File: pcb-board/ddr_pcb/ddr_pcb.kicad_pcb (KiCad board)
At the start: 2 copper layers, 65 x 65 mm, 13 parts, among them U1 RP2040_Zero

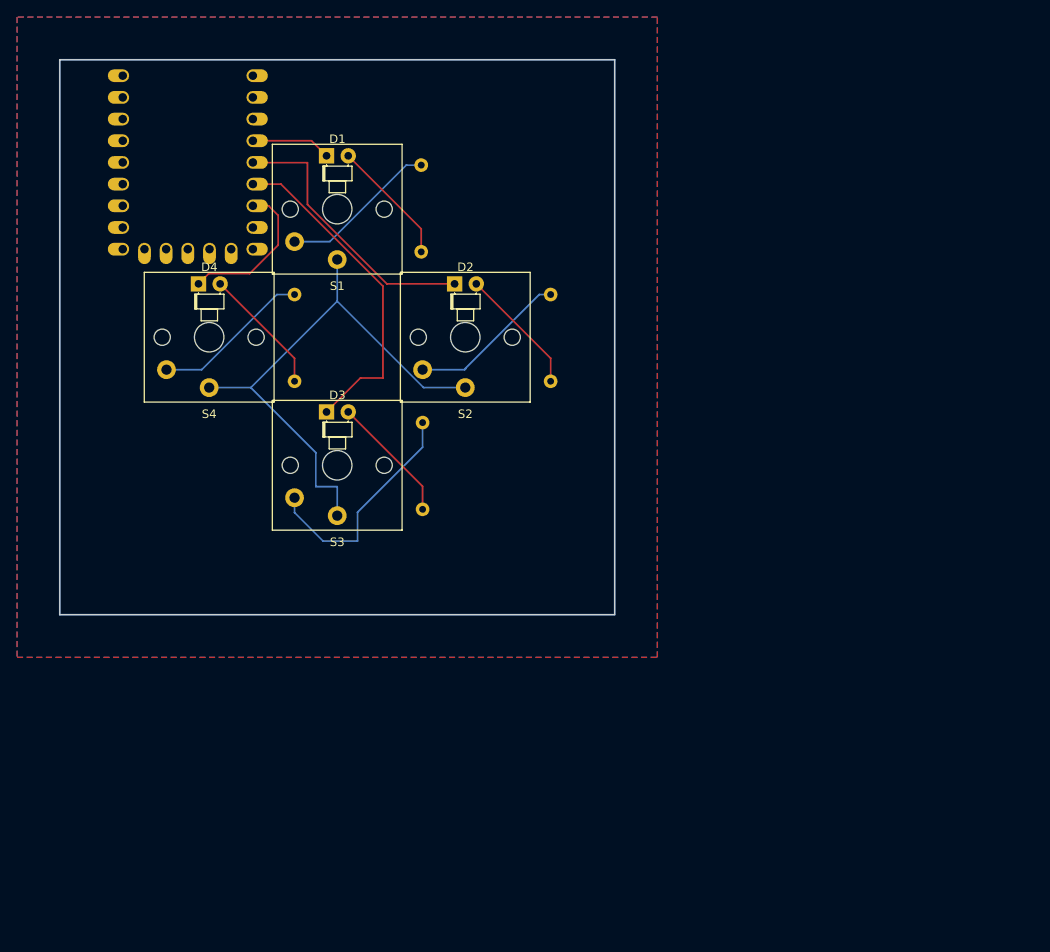
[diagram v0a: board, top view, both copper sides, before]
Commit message: like my 3rd pcb design
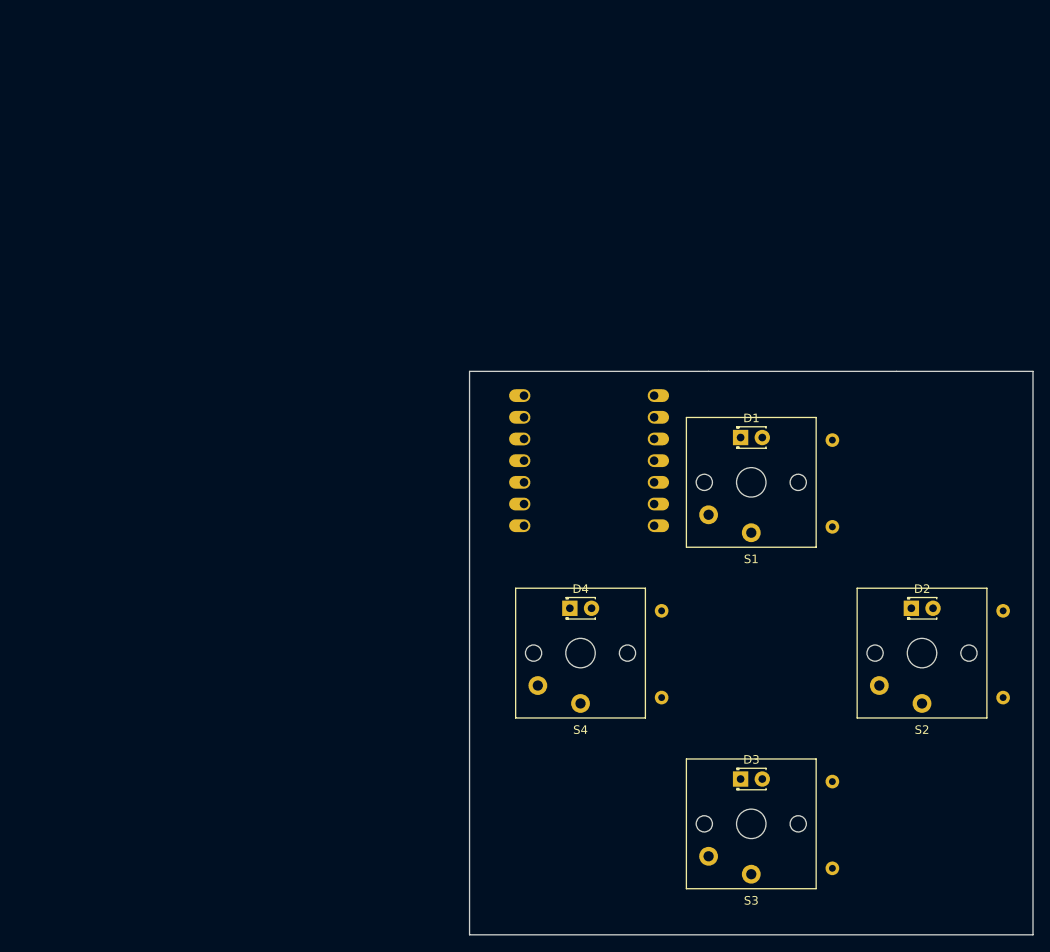
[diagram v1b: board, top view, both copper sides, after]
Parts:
- D1, D2, D3, D4: footprint LED_THT:LED_D1.8mm_W1.8mm_H2.4mm_Horizontal_O1.27mm_Z1.6mm -> LED_THT:LED_D1.8mm_W3.3mm_H2.4mm
- S1, S2, S3, S4: footprint ScottoKeebs_Choc:Choc_V1 -> ScottoKeebs_Choc:Choc_V1_1.00u
- moved D2 65.6 mm to (179.8, 84.2)
- moved S2 65.0 mm to (181.0, 89.5)
- moved D3 64.8 mm to (159.8, 104.2)
- moved S3 64.2 mm to (161.0, 109.5)
- moved U1 60.1 mm to (142.0, 69.5)
- moved R2 59.4 mm to (190.5, 84.5), turned to -90 degrees
- moved D1 58.7 mm to (159.8, 64.2)
- moved S1 58.1 mm to (161.0, 69.5)
- moved D4 57.8 mm to (139.8, 84.2)
- moved R3 57.6 mm to (170.5, 104.5), turned to -90 degrees
- moved S4 57.1 mm to (141.0, 89.5)
- moved R4 56.8 mm to (150.5, 94.7)
- moved R1 53.0 mm to (170.5, 64.5), turned to -90 degrees
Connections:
- D1 pad 1: UP -> GND
- D2 pad 1: RIGHT -> GND
- D3 pad 1: DOWN -> GND
- D4 pad 1: LEFT -> GND
- S1 pad 1: VCC -> UP
- S2 pad 1: VCC -> RIGHT
- S3 pad 1: VCC -> DOWN
- S4 pad 1: VCC -> LEFT
- U1 pad 22: unconnected-(U1-GND-Pad22) -> GND
- U1 pad 23: VCC -> unconnected-(U1-5V-Pad23)
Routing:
- net VCC: track 63.9 -> 0.00 mm
- net DOWN: track 39.2 -> 0.00 mm
- net RIGHT: track 32.4 -> 0.00 mm
- net Net-(R3-Pad2): track 27.5 -> 0.00 mm
- net Net-(R2-Pad2): track 18.7 -> 0.00 mm
- net Net-(R4-Pad2): track 18.6 -> 0.00 mm
- net Net-(R1-Pad2): track 18.6 -> 0.00 mm
- net LEFT: track 18.1 -> 0.00 mm
- net Net-(D2-A): track 15.0 -> 0.00 mm
- net Net-(D3-A): track 15.0 -> 0.00 mm
- net Net-(D4-A): track 15.0 -> 0.00 mm
- net Net-(D1-A): track 14.8 -> 0.00 mm
- net UP: track 9.36 -> 0.00 mm
- removed copper zone on B.Cu, net (none)
- removed copper zone on F.Cu, net (none)
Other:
- board size 65 x 65 mm -> 66 x 66 mm

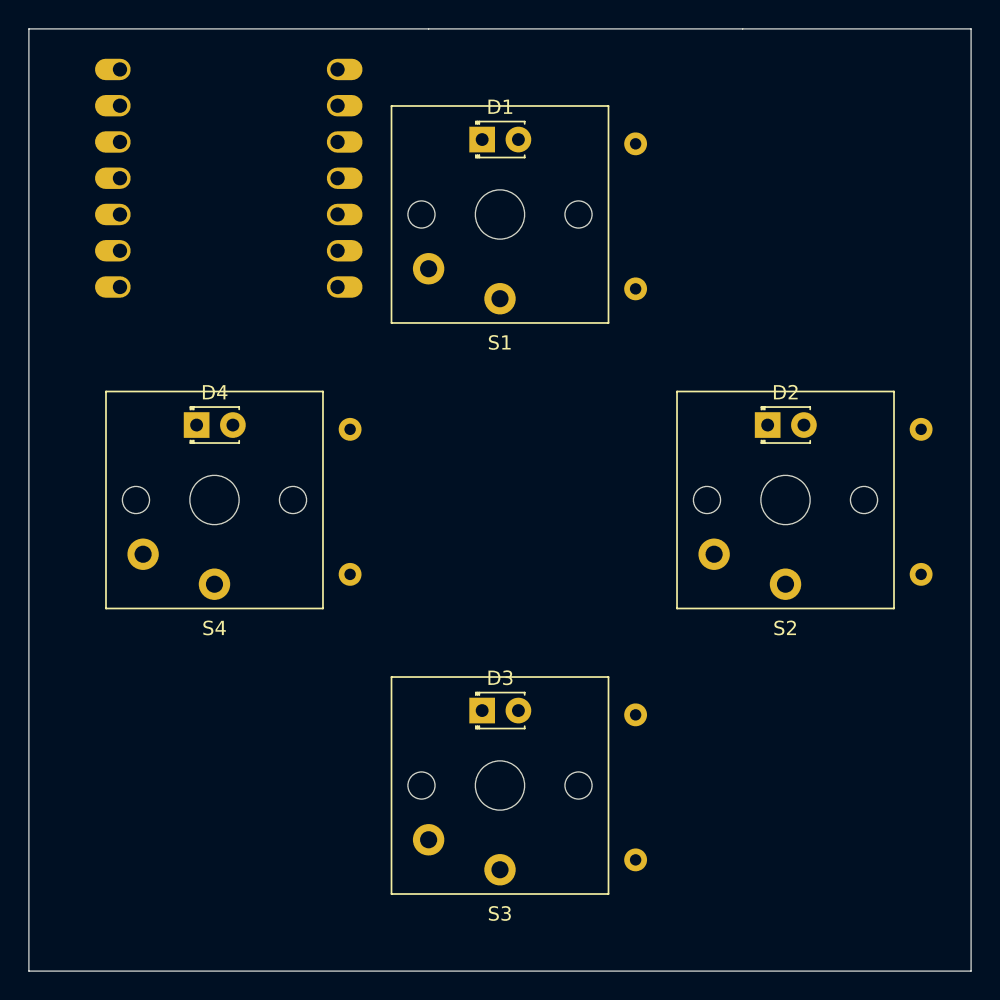
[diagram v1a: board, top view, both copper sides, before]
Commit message: starting code
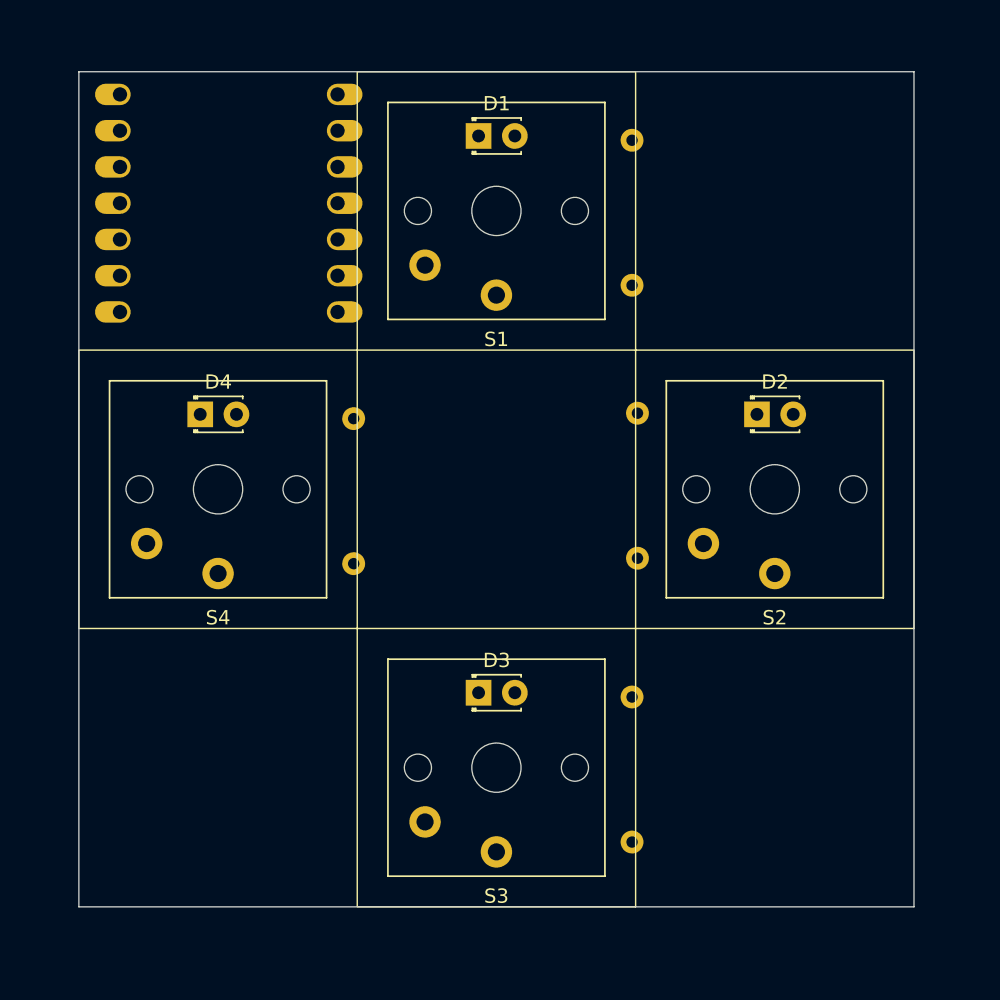
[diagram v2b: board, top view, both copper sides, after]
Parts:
- moved R2 19.9 mm to (170.6, 83.4)
- moved U1 1.75 mm to (142.0, 71.2)
- moved D3 1.27 mm to (159.5, 103.0)
- moved R3 1.27 mm to (170.2, 103.3)
- moved S3 1.27 mm to (160.8, 108.2)
- moved D2 1.06 mm to (179.0, 83.5)
- moved S2 1.06 mm to (180.2, 88.8)
- moved D4 0.79 mm to (140.0, 83.5)
- moved R4 0.79 mm to (150.8, 94.0)
- moved S4 0.79 mm to (141.2, 88.8)
- moved D1 0.35 mm to (159.5, 64.0)
- moved R1 0.35 mm to (170.2, 64.3)
- moved S1 0.35 mm to (160.8, 69.2)
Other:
- board size 66 x 66 mm -> 58.5 x 58.5 mm
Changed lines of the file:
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@@
 	(footprint "ScottoKeebs_Choc:Choc_V1_1.00u"
 		(layer "F.Cu")
-		(at 161 69.5 180)
+		(at 160.75 69.25 180)
 		(descr "Choc keyswitch V1 CPG1350 V1 Keycap 1.00u")
 		(tags "Choc Keyswitch Switch CPG1350 V1 Cutout Keycap 1.00u")
@@
 			(layer "F.SilkS")
 		)
-		(fp_line
-			(start 10 10)
-			(end 10 -10)
-			(stroke
-				(width 0.1)
-				(type solid)
-			)
-			(layer "Dwgs.User")
-		)
-		(fp_line
-			(start 10 -10)
-			(end -10 -10)
-			(stroke
-				(width 0.1)
-				(type solid)
-			)
-			(layer "Dwgs.User")
-		)
-		(fp_line
-			(start -10 10)
-			(end 10 10)
-			(stroke
-				(width 0.1)
-				(type solid)
-			)
-			(layer "Dwgs.User")
-		)
-		(fp_line
-			(start -10 -10)
-			(end -10 10)
+		(fp_rect
+			(start -9.75 -9.75)
+			(end 9.75 9.75)
 			(stroke
 				(width 0.1)
-				(type solid)
+				(type default)
 			)
-			(layer "Dwgs.User")
+			(fill none)
+			(layer "F.SilkS")
 		)
 		(fp_line
@@
 	(footprint "LED_THT:LED_D1.8mm_W3.3mm_H2.4mm"
 		(layer "F.Cu")
-		(at 139.75 84.25)
+		(at 140 83.5)
 		(descr "LED, Round,  Rectangular size 3.3x2.4mm^2 diameter 1.8mm, 2 pins")
 		(tags "LED Round  Rectangular size 3.3x2.4mm^2 diameter 1.8mm 2 pins")
@@
 	(footprint "LED_THT:LED_D1.8mm_W3.3mm_H2.4mm"
 		(layer "F.Cu")
-		(at 159.75 64.25)
+		(at 159.5 64)
 		(descr "LED, Round,  Rectangular size 3.3x2.4mm^2 diameter 1.8mm, 2 pins")
 		(tags "LED Round  Rectangular size 3.3x2.4mm^2 diameter 1.8mm 2 pins")
@@
 	(footprint "ScottoKeebs_Choc:Choc_V1_1.00u"
 		(layer "F.Cu")
-		(at 181 89.5 180)
+		(at 180.25 88.75 180)
 		(descr "Choc keyswitch V1 CPG1350 V1 Keycap 1.00u")
 		(tags "Choc Keyswitch Switch CPG1350 V1 Cutout Keycap 1.00u")
@@
 			(layer "F.SilkS")
 		)
-		(fp_line
-			(start 10 10)
-			(end 10 -10)
-			(stroke
-				(width 0.1)
-				(type solid)
-			)
-			(layer "Dwgs.User")
-		)
-		(fp_line
-			(start 10 -10)
-			(end -10 -10)
-			(stroke
-				(width 0.1)
-				(type solid)
-			)
-			(layer "Dwgs.User")
-		)
-		(fp_line
-			(start -10 10)
-			(end 10 10)
-			(stroke
-				(width 0.1)
-				(type solid)
-			)
-			(layer "Dwgs.User")
-		)
-		(fp_line
-			(start -10 -10)
-			(end -10 10)
+		(fp_rect
+			(start -9.75 -9.75)
+			(end 9.75 9.75)
 			(stroke
 				(width 0.1)
-				(type solid)
+				(type default)
 			)
-			(layer "Dwgs.User")
+			(fill none)
+			(layer "F.SilkS")
 		)
 		(fp_line
@@
 	(footprint "LED_THT:LED_D1.8mm_W3.3mm_H2.4mm"
 		(layer "F.Cu")
-		(at 179.75 84.25)
+		(at 179 83.5)
 		(descr "LED, Round,  Rectangular size 3.3x2.4mm^2 diameter 1.8mm, 2 pins")
 		(tags "LED Round  Rectangular size 3.3x2.4mm^2 diameter 1.8mm 2 pins")
@@
 	(footprint "LED_THT:LED_D1.8mm_W3.3mm_H2.4mm"
 		(layer "F.Cu")
-		(at 159.75 104.25)
+		(at 159.5 103)
 		(descr "LED, Round,  Rectangular size 3.3x2.4mm^2 diameter 1.8mm, 2 pins")
 		(tags "LED Round  Rectangular size 3.3x2.4mm^2 diameter 1.8mm 2 pins")
@@
 	(footprint "ScottoKeebs_Choc:Choc_V1_1.00u"
 		(layer "F.Cu")
-		(at 161 109.5 180)
+		(at 160.75 108.25 180)
 		(descr "Choc keyswitch V1 CPG1350 V1 Keycap 1.00u")
 		(tags "Choc Keyswitch Switch CPG1350 V1 Cutout Keycap 1.00u")
@@
 			(layer "F.SilkS")
 		)
-		(fp_line
-			(start 10 10)
-			(end 10 -10)
-			(stroke
-				(width 0.1)
-				(type solid)
-			)
-			(layer "Dwgs.User")
-		)
-		(fp_line
-			(start 10 -10)
-			(end -10 -10)
-			(stroke
-				(width 0.1)
-				(type solid)
-			)
-			(layer "Dwgs.User")
-		)
-		(fp_line
-			(start -10 10)
-			(end 10 10)
-			(stroke
-				(width 0.1)
-				(type solid)
-			)
-			(layer "Dwgs.User")
-		)
-		(fp_line
-			(start -10 -10)
-			(end -10 10)
+		(fp_rect
+			(start -9.75 -9.75)
+			(end 9.75 9.75)
 			(stroke
 				(width 0.1)
-				(type solid)
+				(type default)
 			)
-			(layer "Dwgs.User")
+			(fill none)
+			(layer "F.SilkS")
 		)
 		(fp_line
@@
 	(footprint "ScottoKeebs_Choc:Choc_V1_1.00u"
 		(layer "F.Cu")
-		(at 141 89.5 180)
+		(at 141.25 88.75 180)
 		(descr "Choc keyswitch V1 CPG1350 V1 Keycap 1.00u")
 		(tags "Choc Keyswitch Switch CPG1350 V1 Cutout Keycap 1.00u")
@@
 			(layer "F.SilkS")
 		)
-		(fp_line
-			(start 10 10)
-			(end 10 -10)
-			(stroke
-				(width 0.1)
-				(type solid)
-			)
-			(layer "Dwgs.User")
-		)
-		(fp_line
-			(start 10 -10)
-			(end -10 -10)
-			(stroke
-				(width 0.1)
-				(type solid)
-			)
-			(layer "Dwgs.User")
-		)
-		(fp_line
-			(start -10 10)
-			(end 10 10)
+		(fp_rect
+			(start -9.75 -9.75)
+			(end 9.75 9.75)
 			(stroke
 				(width 0.1)
-				(type solid)
+				(type default)
 			)
-			(layer "Dwgs.User")
-		)
-		(fp_line
-			(start -10 -10)
-			(end -10 10)
-			(stroke
-				(width 0.1)
-				(type solid)
-			)
-			(layer "Dwgs.User")
+			(fill none)
+			(layer "F.SilkS")
 		)
 		(fp_line
@@
 	(footprint "Resistor_THT:R_Axial_DIN0207_L6.3mm_D2.5mm_P10.16mm_Horizontal"
 		(layer "B.Cu")
-		(at 170.5 104.55 -90)
+		(at 170.25 103.3 -90)
 		(descr "Resistor, Axial_DIN0207 series, Axial, Horizontal, pin pitch=10.16mm, 0.25W = 1/4W, length*diameter=6.3*2.5mm^2, http://cdn-reichelt.de/documents/datenblatt/B400/1_4W%23YAG.pdf")
 		(tags "Resistor Axial_DIN0207 series Axial Horizontal pin pitch 10.16mm 0.25W = 1/4W length 6.3mm diameter 2.5mm")
@@
 	(footprint "Resistor_THT:R_Axial_DIN0207_L6.3mm_D2.5mm_P10.16mm_Horizontal"
 		(layer "B.Cu")
-		(at 190.5 84.55 -90)
+		(at 170.63 83.42 -90)
 		(descr "Resistor, Axial_DIN0207 series, Axial, Horizontal, pin pitch=10.16mm, 0.25W = 1/4W, length*diameter=6.3*2.5mm^2, http://cdn-reichelt.de/documents/datenblatt/B400/1_4W%23YAG.pdf")
 		(tags "Resistor Axial_DIN0207 series Axial Horizontal pin pitch 10.16mm 0.25W = 1/4W length 6.3mm diameter 2.5mm")
@@
 	(footprint "Resistor_THT:R_Axial_DIN0207_L6.3mm_D2.5mm_P10.16mm_Horizontal"
 		(layer "B.Cu")
-		(at 170.5 64.55 -90)
+		(at 170.25 64.3 -90)
 		(descr "Resistor, Axial_DIN0207 series, Axial, Horizontal, pin pitch=10.16mm, 0.25W = 1/4W, length*diameter=6.3*2.5mm^2, http://cdn-reichelt.de/documents/datenblatt/B400/1_4W%23YAG.pdf")
 		(tags "Resistor Axial_DIN0207 series Axial Horizontal pin pitch 10.16mm 0.25W = 1/4W length 6.3mm diameter 2.5mm")
@@
 	(footprint "Resistor_THT:R_Axial_DIN0207_L6.3mm_D2.5mm_P10.16mm_Horizontal"
 		(layer "B.Cu")
-		(at 150.5 94.71 90)
+		(at 150.75 93.96 90)
 		(descr "Resistor, Axial_DIN0207 series, Axial, Horizontal, pin pitch=10.16mm, 0.25W = 1/4W, length*diameter=6.3*2.5mm^2, http://cdn-reichelt.de/documents/datenblatt/B400/1_4W%23YAG.pdf")
 		(tags "Resistor Axial_DIN0207 series Axial Horizontal pin pitch 10.16mm 0.25W = 1/4W length 6.3mm diameter 2.5mm")
@@
 	(footprint "ScottoKeebs_MCU:RP2040_Zero"
 		(layer "B.Cu")
-		(at 142 69.5 180)
+		(at 142 71.25 180)
 		(property "Reference" "U1"
 			(at 0 1.4 0)
@@
 		)
 	)
-	(gr_line
-		(start 128 56.5)
-		(end 156 56.5)
-		(stroke
-			(width 0.05)
-			(type default)
-		)
-		(layer "Edge.Cuts")
-	)
-	(gr_line
-		(start 128 122.5)
-		(end 128 56.5)
-		(stroke
-			(width 0.05)
-			(type default)
-		)
-		(layer "Edge.Cuts")
-	)
-	(gr_line
-		(start 194 56.5)
-		(end 194 122.5)
-		(stroke
-			(width 0.05)
-			(type default)
-		)
-		(layer "Edge.Cuts")
-	)
-	(gr_line
-		(start 156 56.5)
-		(end 178 56.5)
-		(stroke
-			(width 0.05)
-			(type default)
-		)
-		(layer "Edge.Cuts")
-	)
-	(gr_line
-		(start 178 56.5)
-		(end 194 56.5)
-		(stroke
-			(width 0.05)
-			(type default)
-		)
-		(layer "Edge.Cuts")
-	)
-	(gr_line
-		(start 194 122.5)
-		(end 128 122.5)
+	(gr_rect
+		(start 131.5 59.5)
+		(end 190 118)
 		(stroke
 			(width 0.05)
 			(type default)
 		)
+		(fill none)
 		(layer "Edge.Cuts")
 	)
